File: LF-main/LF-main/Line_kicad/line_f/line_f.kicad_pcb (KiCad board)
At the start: 2 copper layers, 135 x 150 mm, 16 parts, among them M2 Motor_DC, M3 Motor_DC, M4 NOT_MOTOR, SW1 SW_SPST, SW2 SW_SPDT, SW3 SW_Push, SW4 SW_Push, U1 TB6612FNG_LINE, m1 BLACKPILL

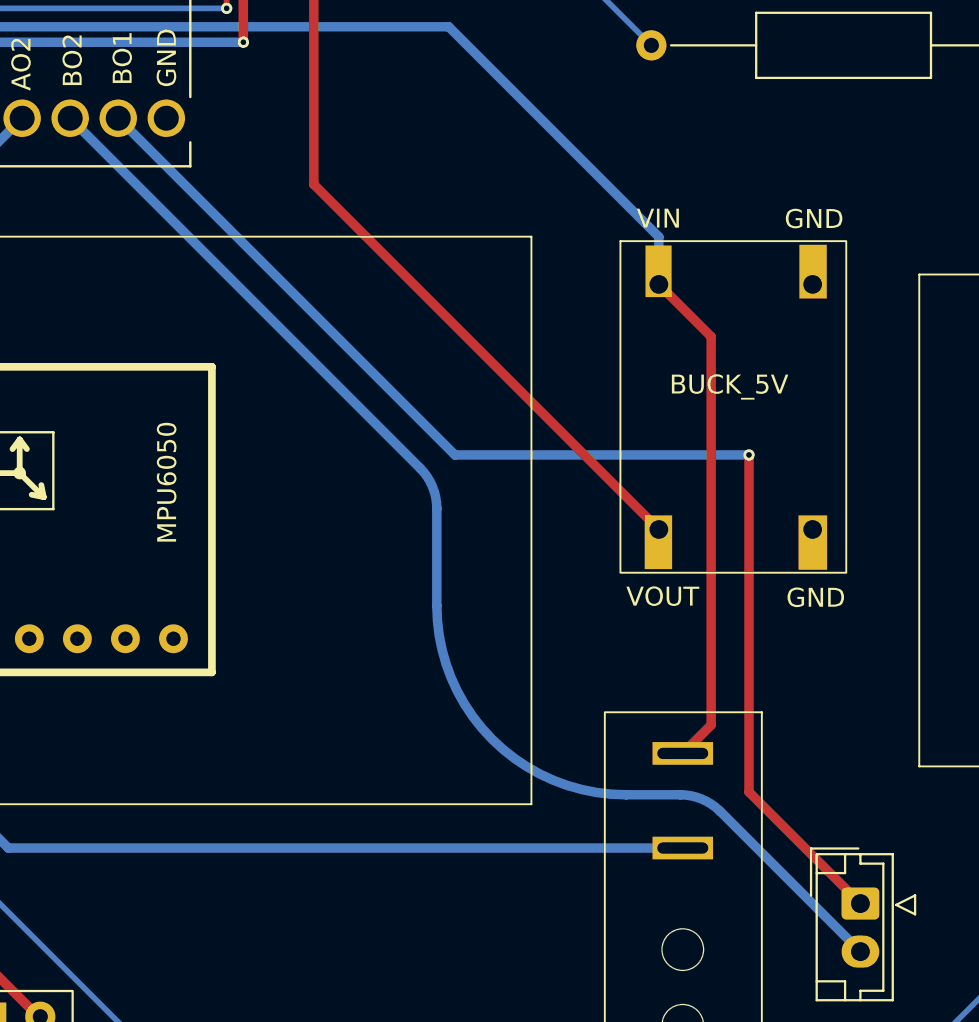
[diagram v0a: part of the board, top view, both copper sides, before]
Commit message: 7r-start.77#
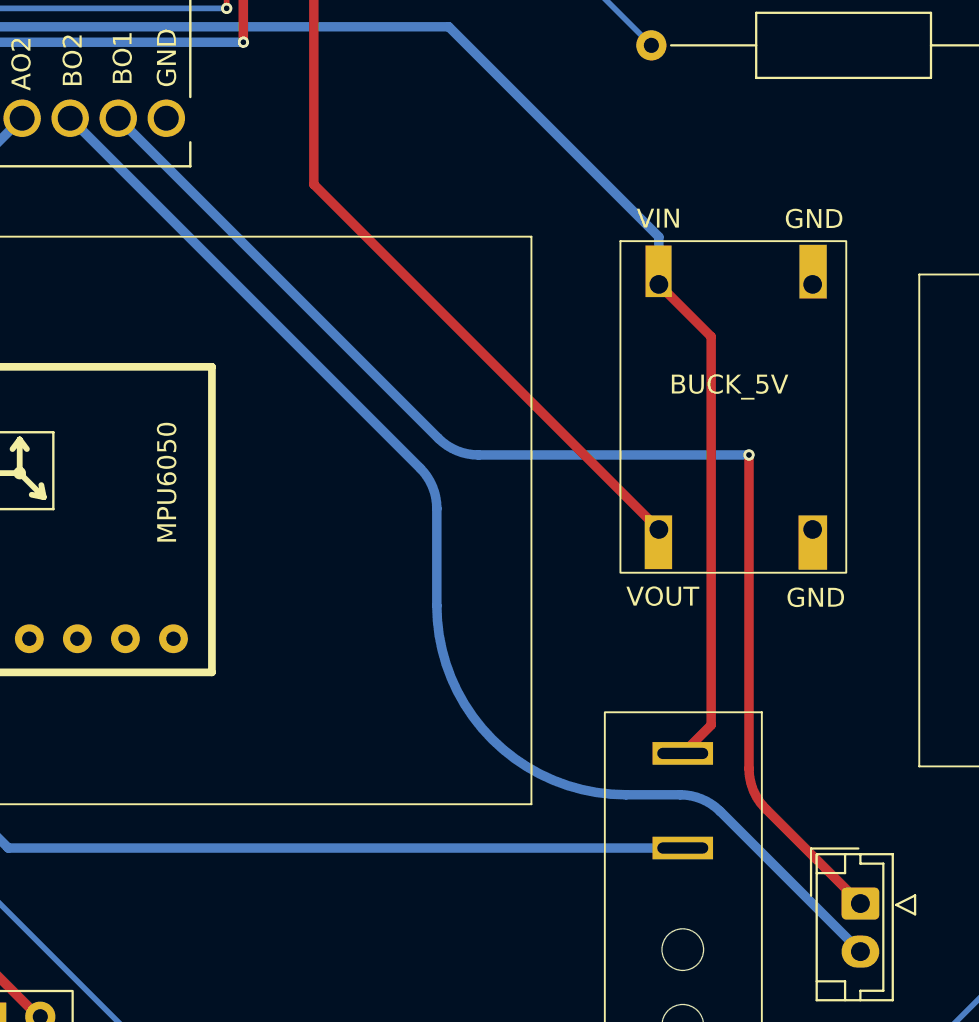
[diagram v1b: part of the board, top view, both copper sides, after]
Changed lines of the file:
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@@
 	)
 	(segment
-		(start 127.5 156.36)
+		(start 128.37868 157.23868)
 		(end 133.39 162.25)
 		(width 0.5)
@@
 	(segment
 		(start 127.5 138.539)
-		(end 127.5 156.36)
+		(end 127.5 155.117359)
 		(width 0.5)
 		(layer "F.Cu")
@@
 		(net 48)
 	)
+	(arc
+		(start 127.5 155.117359)
+		(mid 127.728362 156.26541)
+		(end 128.37868 157.23868)
+		(width 0.5)
+		(layer "F.Cu")
+		(net 48)
+	)
 	(segment
-		(start 111.959 138.539)
+		(start 113.201641 138.539)
 		(end 127.5 138.539)
 		(width 0.5)
@@
 	(segment
 		(start 94.16 120.74)
-		(end 111.959 138.539)
+		(end 111.080321 137.660321)
 		(width 0.5)
 		(layer "B.Cu")
+		(net 48)
+	)
+	(arc
+		(start 113.201641 138.539)
+		(mid 112.053591 138.310639)
+		(end 111.080321 137.660321)
+		(width 0.5)
+		(layer "B.Cu")

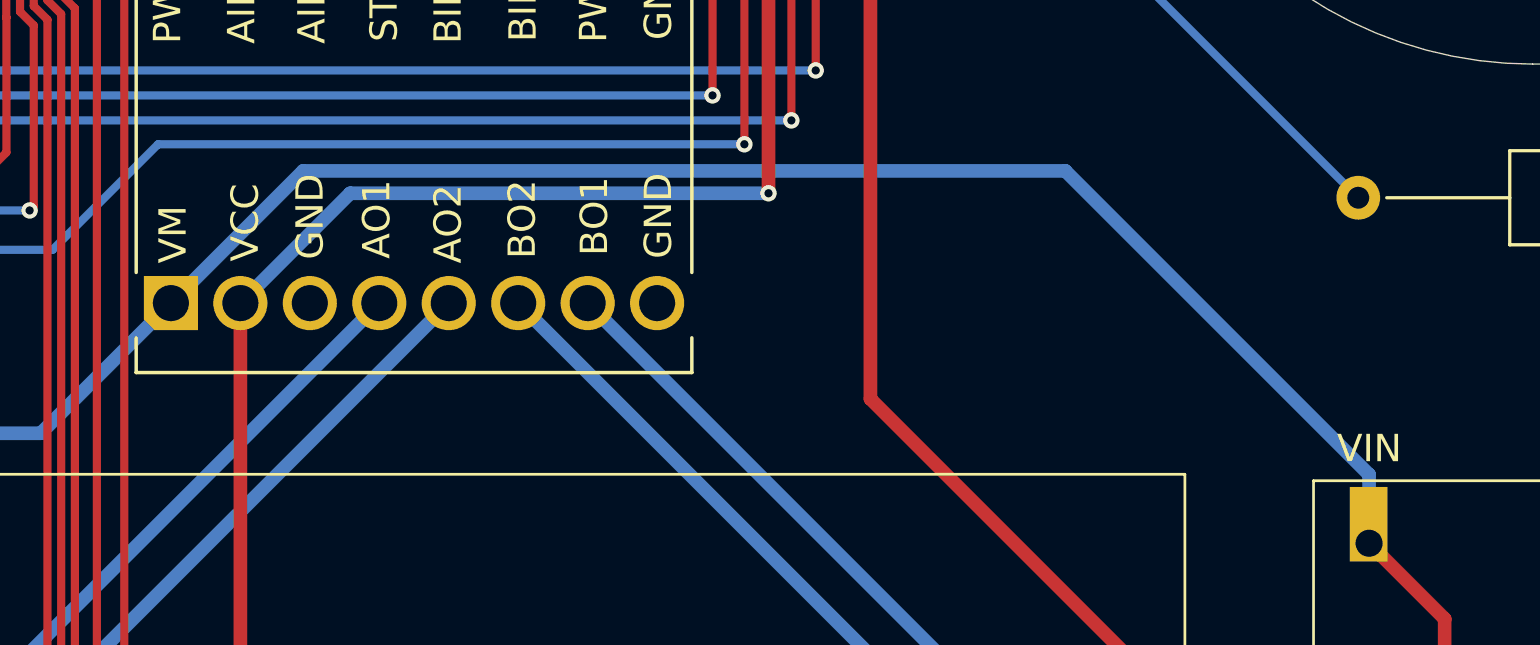
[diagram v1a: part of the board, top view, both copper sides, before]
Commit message: 7r-start.77#
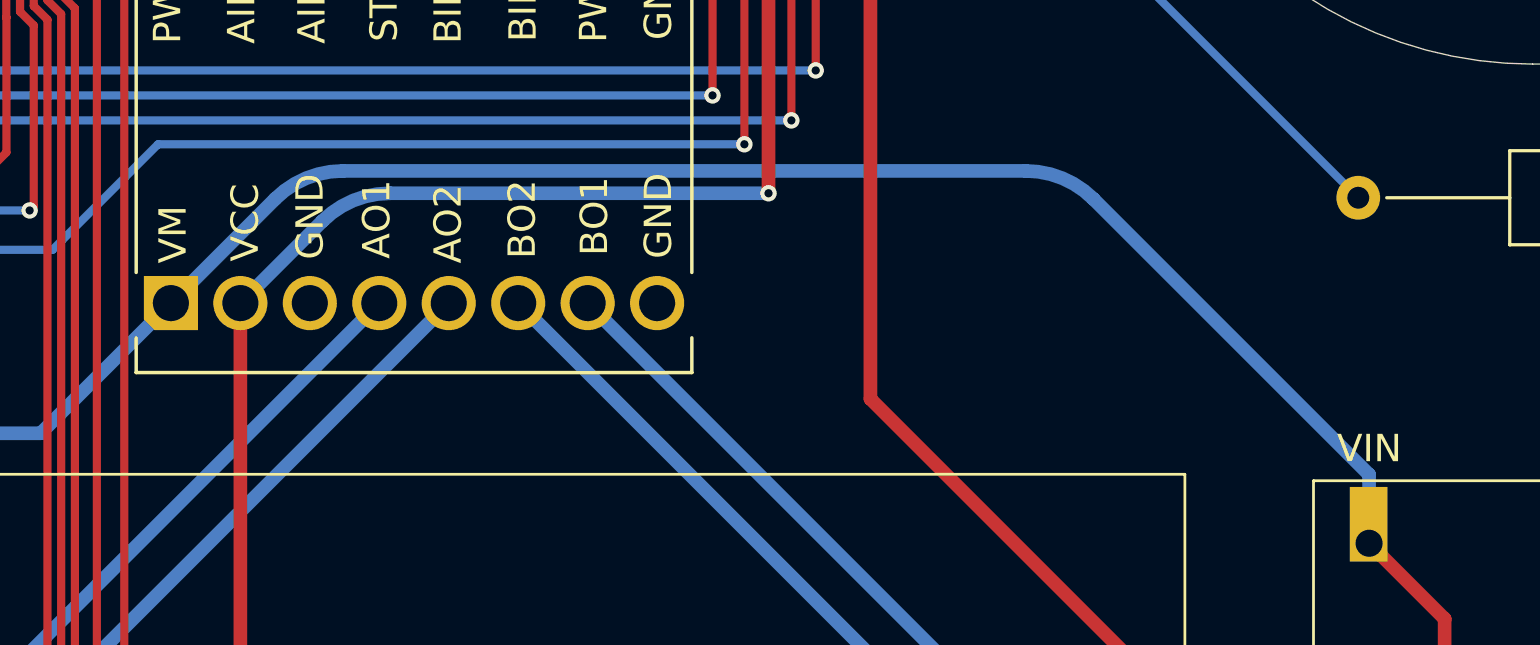
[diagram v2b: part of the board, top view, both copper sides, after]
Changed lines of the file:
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@@
 	(segment
 		(start 122.736 127.011)
-		(end 111.63 115.906)
+		(end 112.655107 116.931015)
 		(width 0.5)
 		(layer "B.Cu")
@@
 	)
 	(segment
-		(start 111.63 115.906)
-		(end 83.7545 115.906)
+		(start 110.180345 115.906)
+		(end 85.204141 115.906)
 		(width 0.5)
 		(layer "B.Cu")
@@
 	)
 	(segment
-		(start 83.7545 115.906)
+		(start 82.729395 116.930999)
 		(end 78.92 120.74)
 		(width 0.5)
@@
 		(net 3)
 	)
+	(arc
+		(start 82.729395 116.930999)
+		(mid 83.864832 116.172387)
+		(end 85.204141 115.906)
+		(width 0.5)
+		(layer "B.Cu")
+		(net 3)
+	)
+	(arc
+		(start 112.655107 116.931015)
+		(mid 111.519664 116.172392)
+		(end 110.180345 115.906)
+		(width 0.5)
+		(layer "B.Cu")
+		(net 3)
+	)
 	(segment
 		(start 95.74 48.74)
@@
 	)
 	(segment
-		(start 85.4773 116.723)
+		(start 86.926971 116.723)
 		(end 100.774 116.723)
 		(width 0.5)
@@
 	(segment
 		(start 81.46 120.74)
-		(end 85.4773 116.723)
-		(width 0.5)
-		(layer "B.Cu")
+		(end 84.45219 117.748034)
+		(width 0.5)
+		(layer "B.Cu")
+		(net 33)
+	)
+	(arc
+		(start 84.45219 117.748034)
+		(mid 85.58764 116.989397)
+		(end 86.926971 116.723)
+		(width 0.5)
+		(layer "B.Cu")
